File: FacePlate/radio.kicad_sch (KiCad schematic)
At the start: 12 parts

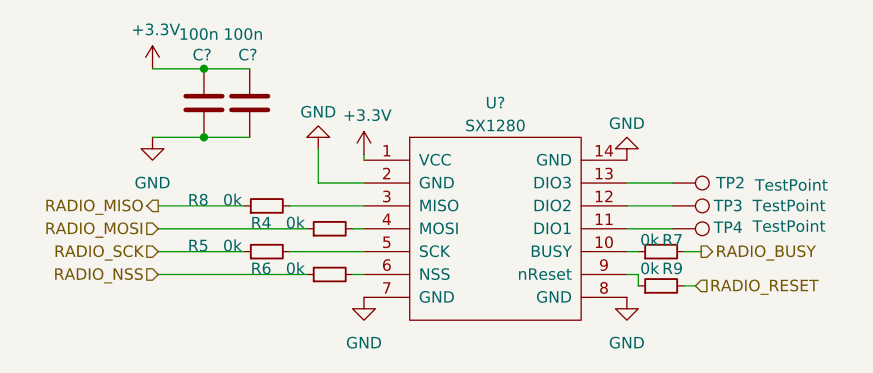
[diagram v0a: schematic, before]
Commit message: faceplate updates
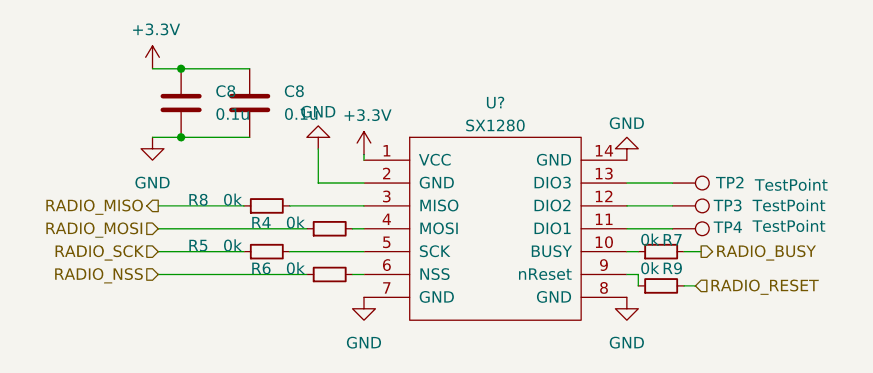
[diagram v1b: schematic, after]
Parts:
- removed C? (x2): 100n, Capacitor_SMD:C_0603_1608Metric, symbol Device:C
- added C8 (x2): 0.1u, bots:C_0603_1608Metric, symbol bots:C_0.1u
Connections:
- net +3.3V: now also C8.1, C8.1
- net GND: now also C8.2, C8.2
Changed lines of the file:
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@@
 (kicad_sch (version 20230121) (generator eeschema)
   (paper "A4")
-  (junction (at 110.49 83.82) (diameter 0) (color 0 0 0 0)
-  )
-  (junction (at 110.49 76.2) (diameter 0) (color 0 0 0 0)
+  (junction (at 107.95 83.82) (diameter 0) (color 0 0 0 0)
+  )
+  (junction (at 107.95 76.2) (diameter 0) (color 0 0 0 0)
+  )
+  (wire (pts (xy 107.95 76.2) (xy 115.57 76.2))
+    (stroke (width 0) (type default))
+  )
+  (wire (pts (xy 107.95 83.82) (xy 115.57 83.82))
+    (stroke (width 0) (type default))
   )
   (wire (pts (xy 123.19 85.09) (xy 123.19 88.9))
     (stroke (width 0) (type default))
   )
-  (wire (pts (xy 104.775 76.2) (xy 110.49 76.2))
+  (wire (pts (xy 104.775 76.2) (xy 107.95 76.2))
     (stroke (width 0) (type default))
   )
@@
     (stroke (width 0) (type default))
   )
-  (wire (pts (xy 110.49 76.2) (xy 115.57 76.2))
-    (stroke (width 0) (type default))
-  )
   (wire (pts (xy 120.015 96.52) (xy 128.27 96.52))
     (stroke (width 0) (type default))
@@
     (stroke (width 0) (type default))
   )
-  (wire (pts (xy 104.775 83.82) (xy 110.49 83.82))
-    (stroke (width 0) (type default))
-  )
   (wire (pts (xy 158.75 99.06) (xy 157.48 99.06))
     (stroke (width 0) (type default))
@@
     (stroke (width 0) (type default))
   )
-  (wire (pts (xy 110.49 83.82) (xy 115.57 83.82))
+  (wire (pts (xy 104.775 83.82) (xy 107.95 83.82))
     (stroke (width 0) (type default))
   )
@@
   (hierarchical_label "RADIO_RESET" (shape input) (at 165.1 100.33 0) (fields_autoplaced)
     (effects (font (size 1.27 1.27)) (justify left))
+  )
+  (symbol (lib_id "bots:C_0.1u") (at 107.95 80.01 0) (unit 1)
+    (in_bom yes) (on_board yes) (dnp no) (fields_autoplaced)
+    (property "Reference" "C8" (at 111.76 78.74 0)
+      (effects (font (size 1.27 1.27)) (justify left))
+    )
+    (property "Value" "0.1u" (at 111.76 81.28 0)
+      (effects (font (size 1.27 1.27)) (justify left))
+    )
+    (property "Footprint" "bots:C_0603_1608Metric" (at 108.9152 83.82 0)
+      (effects (font (size 1.27 1.27)) hide)
+    )
+    (property "Datasheet" "~" (at 107.95 80.01 0)
+      (effects (font (size 1.27 1.27)) hide)
+    )
+    (pin "1")
+    (pin "2")
+    (instances
+      (project "FacePlate"
+        (path "/e63e39d7-6ac0-4ffd-8aa3-1841a4541b55/99bd3b0c-5cef-43ec-97f5-6b19c715565b"
+          (reference "C8") (unit 1)
+        )
+        (path "/e63e39d7-6ac0-4ffd-8aa3-1841a4541b55/e8e72004-885a-48f0-be5d-3ccbb5e9b4ac"
+          (reference "C11") (unit 1)
+        )
+      )
+    )
   )
   (symbol (lib_id "power:GND") (at 128.27 101.6 0) (unit 1)
@@
     )
   )
-  (symbol (lib_id "Device:C") (at 115.57 80.01 0) (unit 1)
-    (in_bom yes) (on_board yes) (dnp no)
-    (property "Reference" "C?" (at 114.3 74.676 0)
-      (effects (font (size 1.27 1.27)) (justify left))
-    )
-    (property "Value" "100n" (at 112.649 72.39 0)
-      (effects (font (size 1.27 1.27)) (justify left))
-    )
-    (property "Footprint" "Capacitor_SMD:C_0603_1608Metric" (at 116.5352 83.82 0)
+  (symbol (lib_id "bots:C_0.1u") (at 115.57 80.01 0) (unit 1)
+    (in_bom yes) (on_board yes) (dnp no) (fields_autoplaced)
+    (property "Reference" "C8" (at 119.38 78.74 0)
+      (effects (font (size 1.27 1.27)) (justify left))
+    )
+    (property "Value" "0.1u" (at 119.38 81.28 0)
+      (effects (font (size 1.27 1.27)) (justify left))
+    )
+    (property "Footprint" "bots:C_0603_1608Metric" (at 116.5352 83.82 0)
       (effects (font (size 1.27 1.27)) hide)
     )
@@
       (effects (font (size 1.27 1.27)) hide)
     )
-    (property "LCSC" "C14663" (at 114.3 84.836 0)
-      (effects (font (size 1.27 1.27)) (justify left) hide)
-    )
-    (pin "1")
-    (pin "2")
-    (instances
-      (project "BoardyMcBoardFace"
-        (path "/ce9c697a-7c8e-40f4-9393-5cd88edd7734"
-          (reference "C?") (unit 1)
-        )
-      )
-      (project "FacePlate"
-        (path "/e63e39d7-6ac0-4ffd-8aa3-1841a4541b55"
-          (reference "C?") (unit 1)
-        )
-        (path "/e63e39d7-6ac0-4ffd-8aa3-1841a4541b55/e8e72004-885a-48f0-be5d-3ccbb5e9b4ac"
-          (reference "C11") (unit 1)
+    (pin "1")
+    (pin "2")
+    (instances
+      (project "FacePlate"
+        (path "/e63e39d7-6ac0-4ffd-8aa3-1841a4541b55/99bd3b0c-5cef-43ec-97f5-6b19c715565b"
+          (reference "C8") (unit 1)
+        )
+        (path "/e63e39d7-6ac0-4ffd-8aa3-1841a4541b55/e8e72004-885a-48f0-be5d-3ccbb5e9b4ac"
+          (reference "C10") (unit 1)
         )
       )
@@
         )
       )
-    )
-  )
-  (symbol (lib_id "Device:C") (at 110.49 80.01 0) (unit 1)
-    (in_bom yes) (on_board yes) (dnp no)
-    (property "Reference" "C?" (at 109.22 74.676 0)
-      (effects (font (size 1.27 1.27)) (justify left))
-    )
-    (property "Value" "100n" (at 107.696 72.39 0)
-      (effects (font (size 1.27 1.27)) (justify left))
-    )
-    (property "Footprint" "Capacitor_SMD:C_0603_1608Metric" (at 111.4552 83.82 0)
-      (effects (font (size 1.27 1.27)) hide)
-    )
-    (property "Datasheet" "~" (at 110.49 80.01 0)
-      (effects (font (size 1.27 1.27)) hide)
-    )
-    (property "LCSC" "C14663" (at 109.22 84.836 0)
-      (effects (font (size 1.27 1.27)) (justify left) hide)
-    )
-    (pin "1")
-    (pin "2")
-    (instances
-      (project "BoardyMcBoardFace"
-        (path "/ce9c697a-7c8e-40f4-9393-5cd88edd7734"
-          (reference "C?") (unit 1)
-        )
-      )
-      (project "FacePlate"
-        (path "/e63e39d7-6ac0-4ffd-8aa3-1841a4541b55"
-          (reference "C?") (unit 1)
-        )
-        (path "/e63e39d7-6ac0-4ffd-8aa3-1841a4541b55/e8e72004-885a-48f0-be5d-3ccbb5e9b4ac"
-          (reference "C10") (unit 1)
-        )
-      )
